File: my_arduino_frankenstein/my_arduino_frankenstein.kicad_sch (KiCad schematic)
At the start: 48 parts, among them J1 Conn_02x03_Odd_Even, J4 Conn_01x04_Pin, J5 Conn_01x04_Pin, J7 Conn_01x04_Pin, U1 LM358, U2 NCP115AMX250TCG, U3 CH340G, U4 TSV994, U5 ATmega328P-M, U7 LM358M

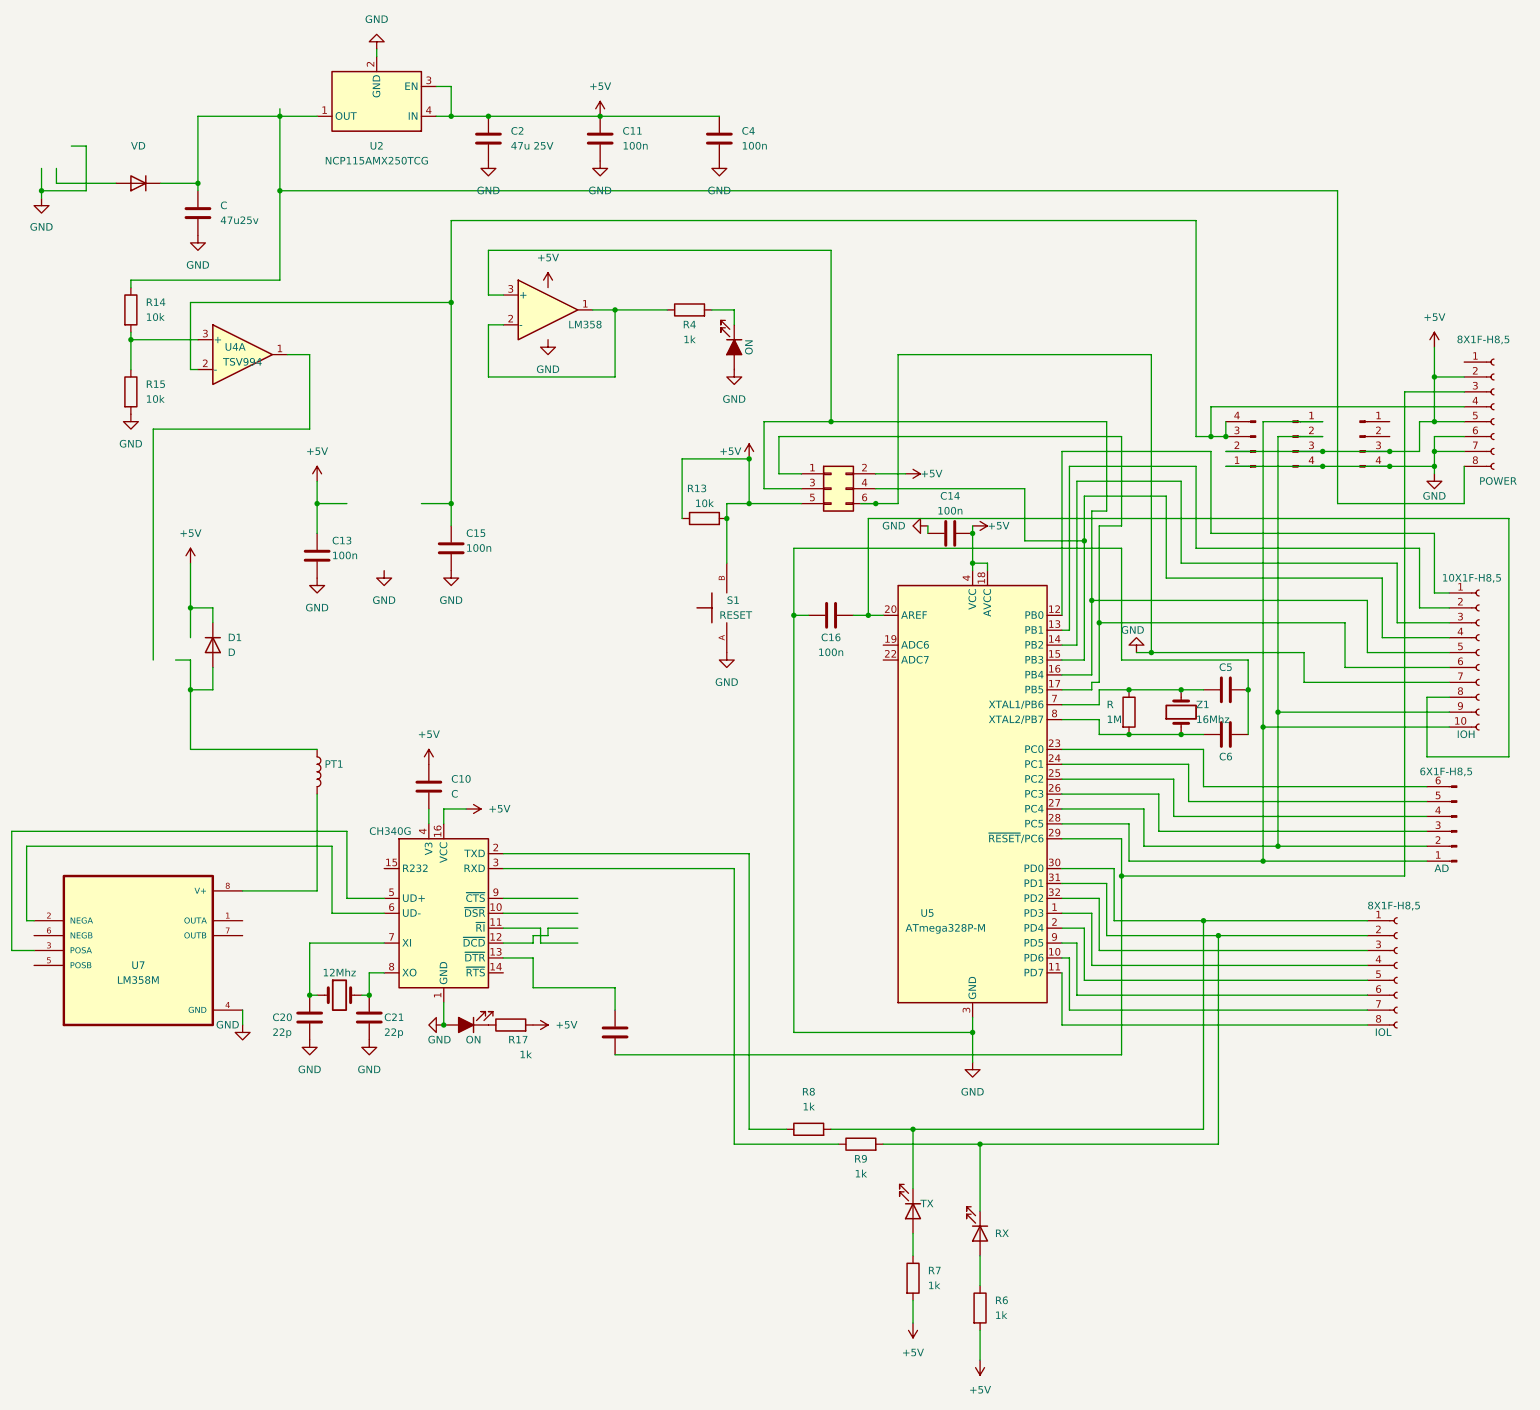
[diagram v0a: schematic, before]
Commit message: final schematics for compact board
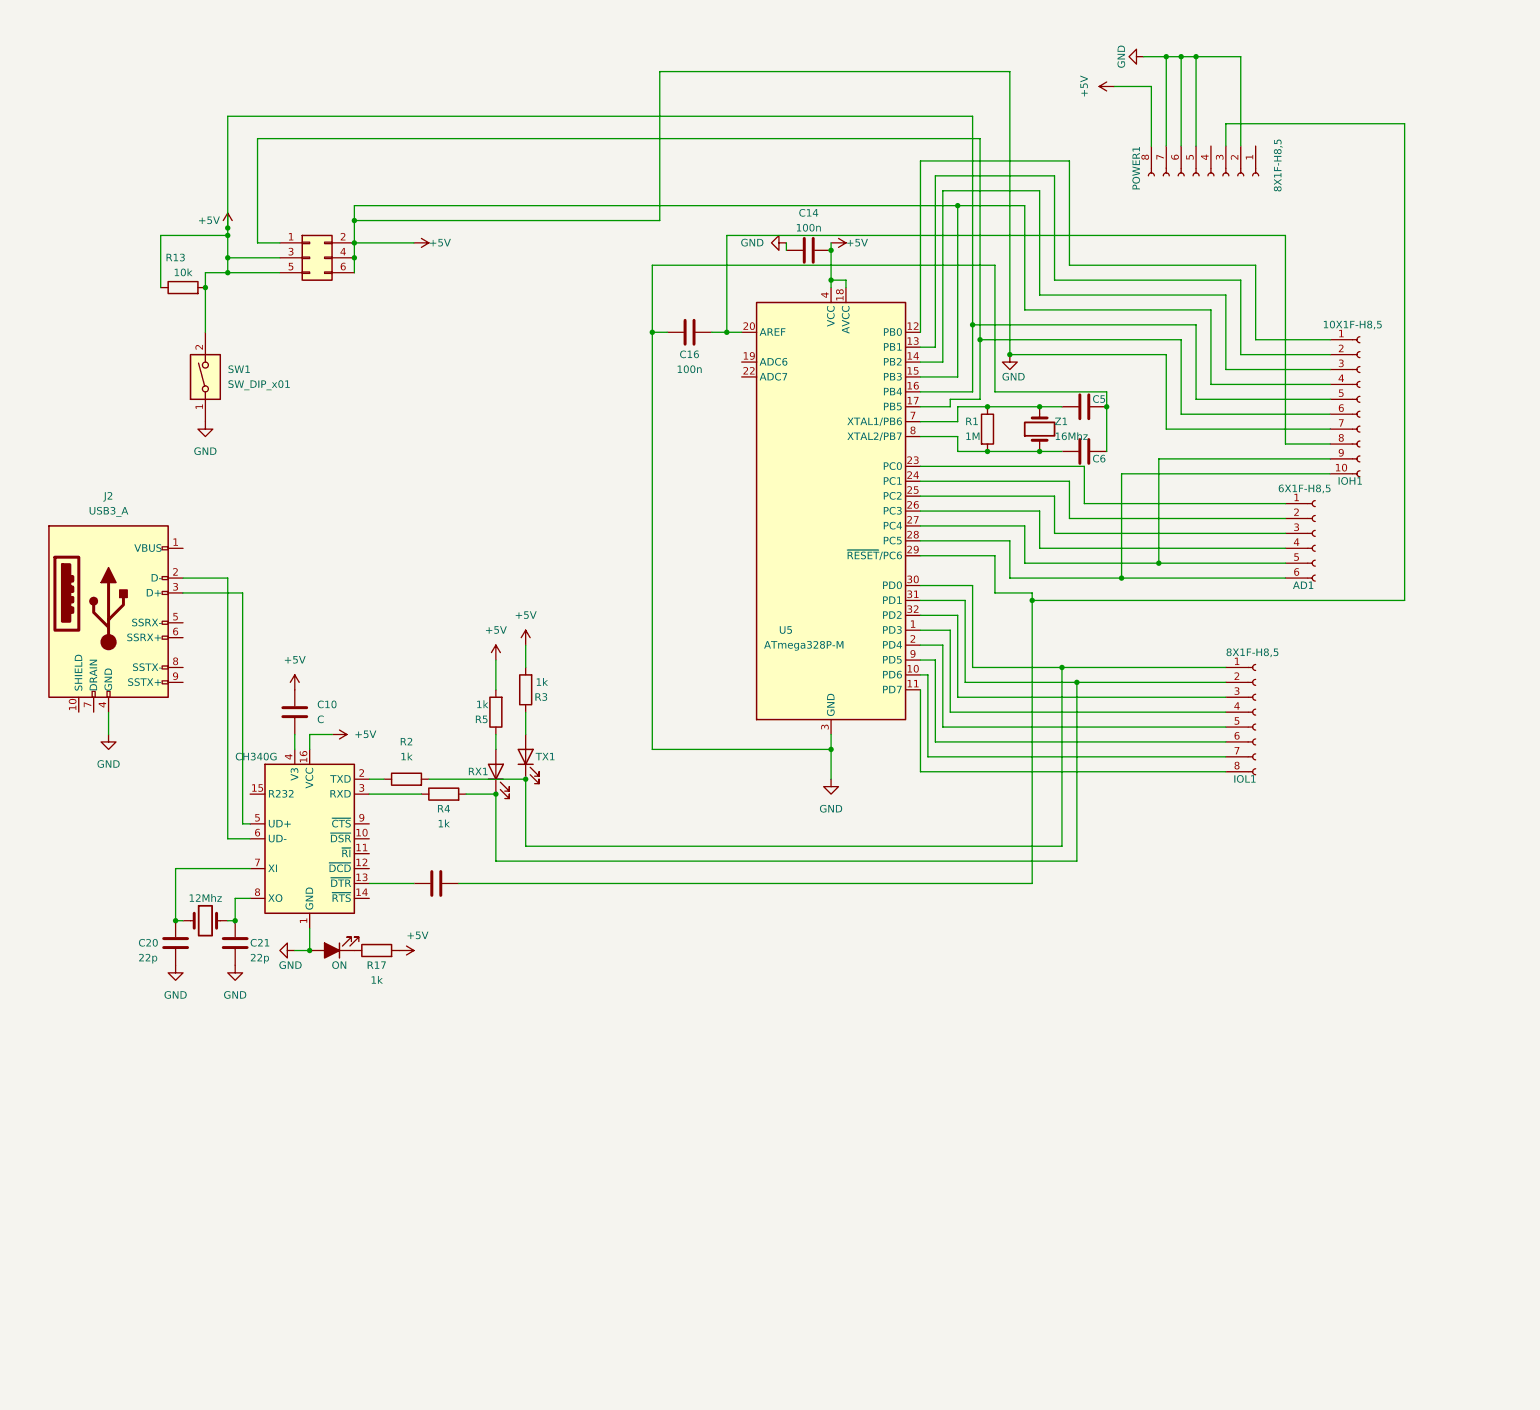
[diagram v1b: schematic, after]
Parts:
- removed AD: 6X1F-H8,5, symbol Connector:Conn_01x06_Pin
- removed C: 47u25v, symbol Device:C
- removed C11, C13, C15, C4: 100n, symbol Device:C
- removed C2: 47u 25V, symbol Device:C
- removed D1, VD: D, symbol Device:D
- removed D3: ON, symbol Device:LED_Filled
- removed J4, J5, J7: Conn_01x04_Pin, symbol Connector:Conn_01x04_Pin
- removed PT1: L, symbol Device:L
- removed R14, R15: 10k, symbol Device:R
- removed R6, R7, R8, R9: 1k, symbol Device:R
- removed RX, TX: LED, symbol Device:LED
- removed S1: RESET, EVQ-PF008K:RIGHTANGLE-PUSHBUTTON, symbol EVQ-PF008K:EVQ-PF008K
- removed U1: LM358, symbol Amplifier_Operational:LM358
- removed U2: NCP115AMX250TCG, Package_DFN_QFN:OnSemi_XDFN4-1EP_1.0x1.0mm_EP0.52x0.52mm, symbol Regulator_Linear:NCP115AMX250TCG
- removed U4: TSV994, symbol Amplifier_Operational:TSV994
- removed U7: LM358M, LM358M:SOIC127P599X175-8N, symbol LM358M:LM358M
- added AD1: 6X1F-H8,5, Connector_PinSocket_1.27mm:PinSocket_1x06_P1.27mm_Vertical, symbol Connector:Conn_01x06_Socket
- added J2: USB3_A, Connector_USB:USB3_A_Molex_48393-001, symbol Connector:USB3_A
- added R2, R3, R5: 1k, Resistor_SMD:R_0201_0603Metric, symbol Device:R
- added RX1, TX1: LED, LED_SMD:LED-APA102-2020, symbol Device:LED
- added SW1: SW_DIP_x01, Button_Switch_SMD:Nidec_Copal_CAS-120A, symbol Switch:SW_DIP_x01
- C1, C10, C14, C16, C20, C21, C5, C6: footprint (none) -> Capacitor_SMD:CP_Elec_3x5.3
- D2: footprint (none) -> LED_SMD:LED-APA102-2020
- IOH1: renamed from IOH; footprint (none) -> Connector_PinSocket_1.27mm:PinSocket_1x10_P1.27mm_Vertical
- IOL1: renamed from IOL; footprint (none) -> Connector_PinHeader_2.54mm:PinHeader_1x08_P2.54mm_Vertical
- J1: footprint (none) -> Connector_PinHeader_2.00mm:PinHeader_2x03_P2.00mm_Vertical
- POWER1: renamed from POWER; footprint (none) -> Connector_PinSocket_2.00mm:PinSocket_1x08_P2.00mm_Vertical
- R1: renamed from R; footprint (none) -> Resistor_SMD:R_0201_0603Metric
- R13, R17, R4: footprint (none) -> Resistor_SMD:R_0201_0603Metric
- Y1: renamed from Y; footprint (none) -> Crystal:Crystal_AT310_D3.0mm_L10.0mm_Horizontal
- Z1: footprint (none) -> Crystal:Crystal_AT310_D3.0mm_L10.0mm_Horizontal
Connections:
- net GND is gone; now on net +5V: C14.1, C16.1, C20.2, C21.2, C5.2, C6.2, D2.2 (A), IOH1.7 (Pin_7), J1.6 (Pin_6), POWER1.6 (Pin_6), POWER1.7 (Pin_7), U3.1 (GND), U5.21 (GND), U5.3 (GND), U5.33 (GND), U5.5 (GND)
- net +5V: now also IOH1.4 (Pin_4), IOH1.5 (Pin_5), J1.3 (Pin_3), J1.4 (Pin_4), POWER1.8 (Pin_8), U5.15 (PB3), U5.16 (PB4), J2.4 (GND), R3.2, R5.2, SW1.1, SW1.2
- net at IOL1.2 (Pin_2), U5.31 (PD1): now also R4.2, RX1.1 (K)
- net at IOL1.1 (Pin_1), U5.30 (PD0): now also R2.2, TX1.1 (K)
- net at IOH1.10 (Pin_10), U5.28 (PC5): now also AD1.6 (Pin_6)
- net at IOH1.9 (Pin_9), U5.27 (PC4): now also AD1.5 (Pin_5)
- net at U5.23 (PC0): now also AD1.1 (Pin_1)
- net at U5.24 (PC1): now also AD1.2 (Pin_2)
- net at U5.25 (PC2): now also AD1.3 (Pin_3)
- net at U5.26 (PC3): now also AD1.4 (Pin_4)
- net at U3.6 (UD-): now also J2.2 (D-)
- net at U3.5 (UD+): now also J2.3 (D+)
- net at U3.3 (RXD): now also R4.1
- net at U3.2 (TXD): now also R2.1
- new net: R5.1, RX1.2 (A)
- new net: R3.1, TX1.2 (A)
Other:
- moved on the sheet: C10, C14, C16, C20, C21, C5, C6, IOH1, IOL1, POWER1, R1, R13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
